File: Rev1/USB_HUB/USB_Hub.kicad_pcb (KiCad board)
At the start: 4 copper layers, 95.9 x 90.2 mm, 79 parts, among them IC1 TLV76733DGNR, IC2 TLV76733DGNR, IC3 USB2513B_M2, IC4 USB2513B_M2, J1 826629-4, J2 826629-4, J4 F3311A7H121014E200, J6 B4B-XH-A, J9 B4B-XH-A, Q1 IRLML2244TRPBF, Q2 IRLML2244TRPBF, Q3 IRLML2244TRPBF, Q4 IRLML2244TRPBF, Q5 IRLML2244TRPBF, Q7 IRLML2244TRPBF, Y1 24MHZ, Y3 24MHZ

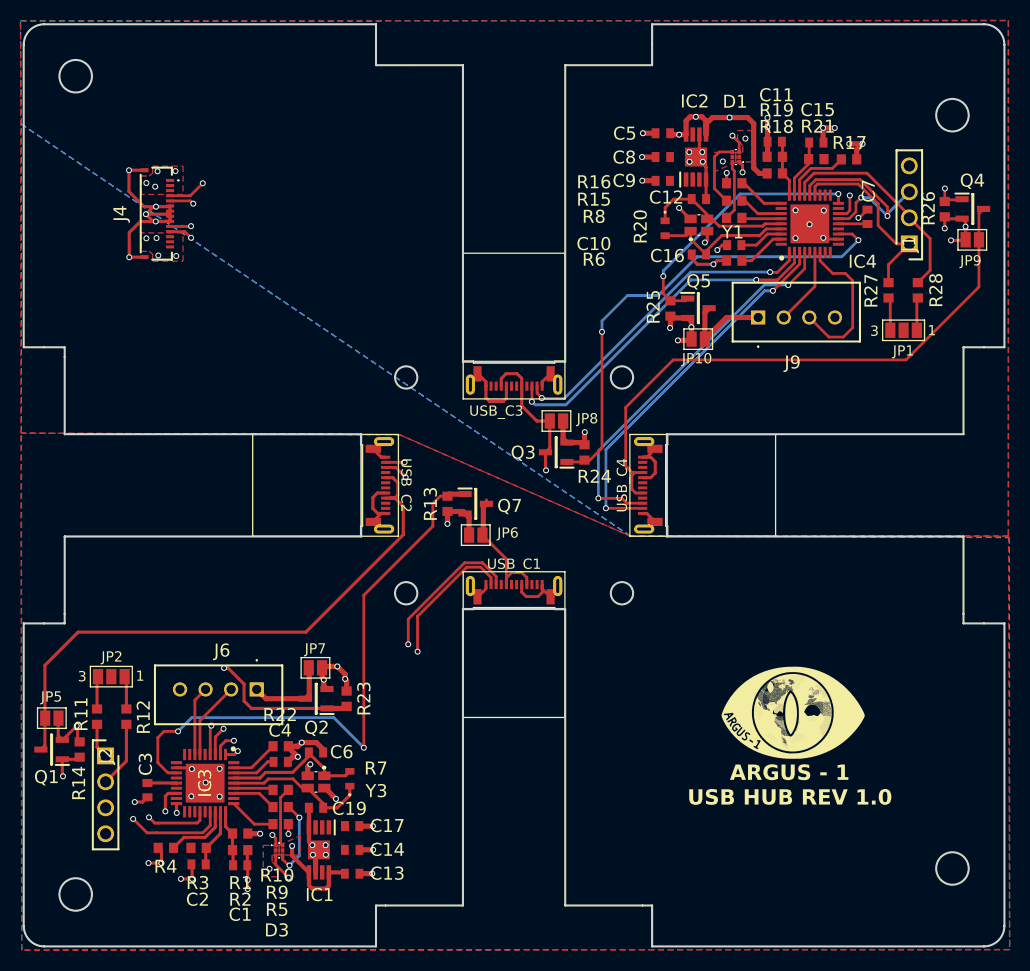
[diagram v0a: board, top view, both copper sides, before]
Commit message: USB HUB Finalized
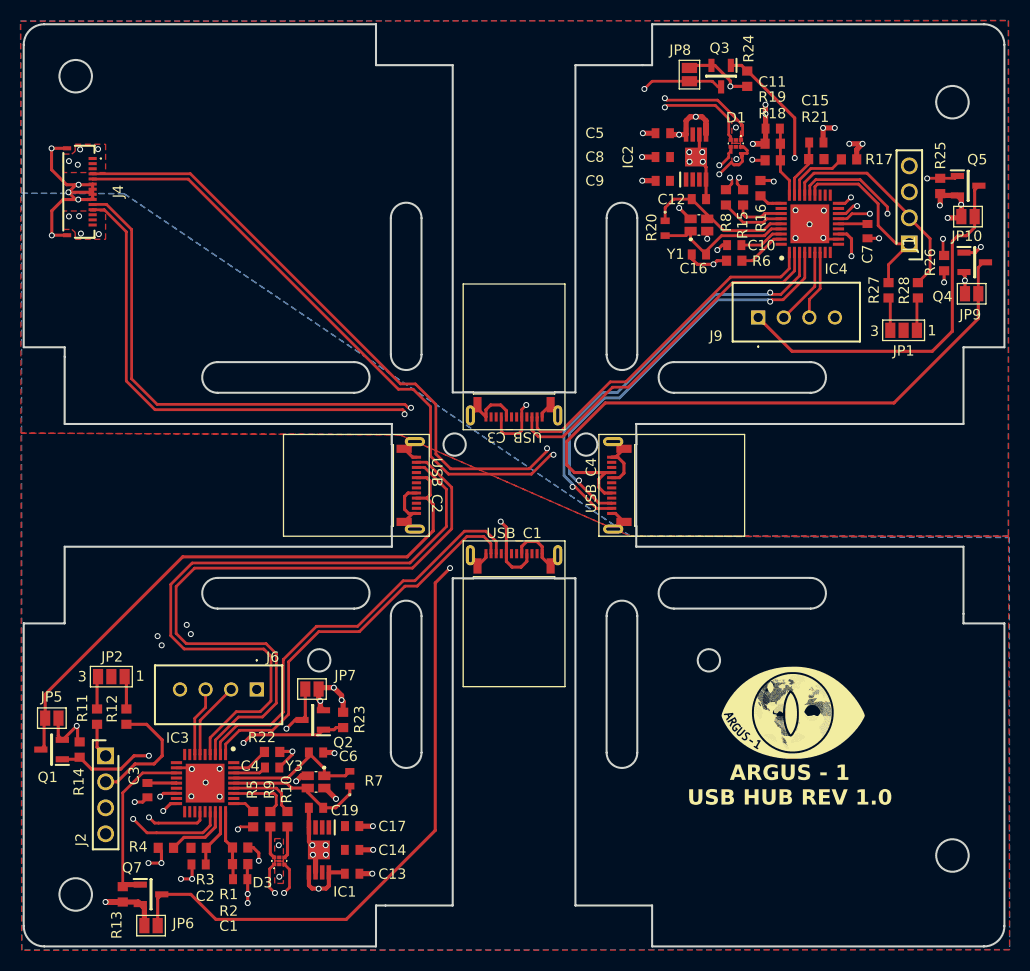
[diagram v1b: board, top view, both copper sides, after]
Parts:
- moved JP6 49.7 mm to (113.5, 139.0)
- moved Q7 49.7 mm to (113.5, 135.9)
- moved R13 49.7 mm to (110.7, 135.9)
- moved Q3 40.2 mm to (169.2, 55.9), turned to -90 degrees
- moved R24 39.9 mm to (171.8, 56.2), turned to 90 degrees
- moved JP8 36.3 mm to (166.1, 55.8), turned to 90 degrees
- moved JP10 29.0 mm to (193.3, 69.7)
- moved Q5 29.0 mm to (193.4, 66.7)
- moved R25 29.0 mm to (190.6, 66.7)
- moved J4 7.87 mm to (106.4, 67.2)
- moved R26 5.27 mm to (191.0, 74.2)
- moved JP9 5.27 mm to (193.7, 77.2)
- moved Q4 5.22 mm to (194.0, 74.2)
- moved USB_C4 3.03 mm to (158.5, 96.0)
- moved USB_C1 3.01 mm to (149.0, 102.6)
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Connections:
- net Net-(D1-input/output_1_1) renamed /Upstream/P2+
- net Net-(D1-input/output_2_1) renamed /Upstream/P2-
- net Net-(IC3-USBDM_UP) renamed /hub_1/1-
- net Net-(IC3-USBDP_UP) renamed /hub_1/1+
- net Net-(IC4-USBDM_UP) renamed /hub_2/2-
- net Net-(IC4-USBDP_UP) renamed /hub_2/2+
- D3 pad 1: Net-(D3-input/output_1_1) -> /Upstream/P1-
- D3 pad 3: Net-(D3-input/output_2_1) -> /Upstream/P1+
- D3 pad 4: D_N_1 -> D_1_P
- D3 pad 6: D_P_1 -> D_1_N
- J4 pad 10: Net-(D3-input/output_2_1) -> /Upstream/P1-
- J4 pad 11: Net-(D3-input/output_1_1) -> /Upstream/P1+
- R10 pad 1: D_P_1 -> D_1_P
- R9 pad 1: D_N_1 -> D_1_N
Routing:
- net /Upstream/P1-: track 0.00 -> 113.6 mm, vias 0 -> 2
- net /Upstream/P1+: track 0.00 -> 111.0 mm, vias 0 -> 2
- net Net-(D3-input/output_2_1): track 93.0 -> 0.00 mm, vias 2 -> 0
- net Net-(D3-input/output_1_1): track 78.8 -> 0.00 mm, vias 2 -> 0
- net Net-(JP6-A): track 13.3 -> 76.4 mm, vias 0 -> 2
- net PRTPWR1: track 57.1 -> 17.0 mm, vias 2 -> 0
- net Net-(JP8-A): track 14.2 -> 52.7 mm, vias 1 -> 2
- net Net-(JP10-A): track 9.29 -> 37.0 mm
- net PORT2_P: track 38.6 -> 65.9 mm, vias 2 -> 0
- net PORT2_N: track 40.3 -> 66.7 mm, vias 2 -> 0
- net /Upstream/P2+: track 84.9 -> 110.3 mm
- net /Upstream/P2-: track 89.0 -> 109.1 mm
- net PRTPWR4: track 47.0 -> 27.4 mm
- net PRTPWR6: track 26.2 -> 12.7 mm
- net PRTPWR3: track 35.8 -> 22.6 mm
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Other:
- outline, holes or cut-outs redrawn
